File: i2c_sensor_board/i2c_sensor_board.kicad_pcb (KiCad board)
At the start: 2 copper layers, 18 parts, among them J1 Conn_01x03_Pin, J2 Conn_01x04_Pin, J3 Conn_01x04_Pin, SW1 SW_Push, U1 STM32G030K8Tx, U2 BME280, U3 TLV75533PDBV, U4 SN74LV1T34DBV

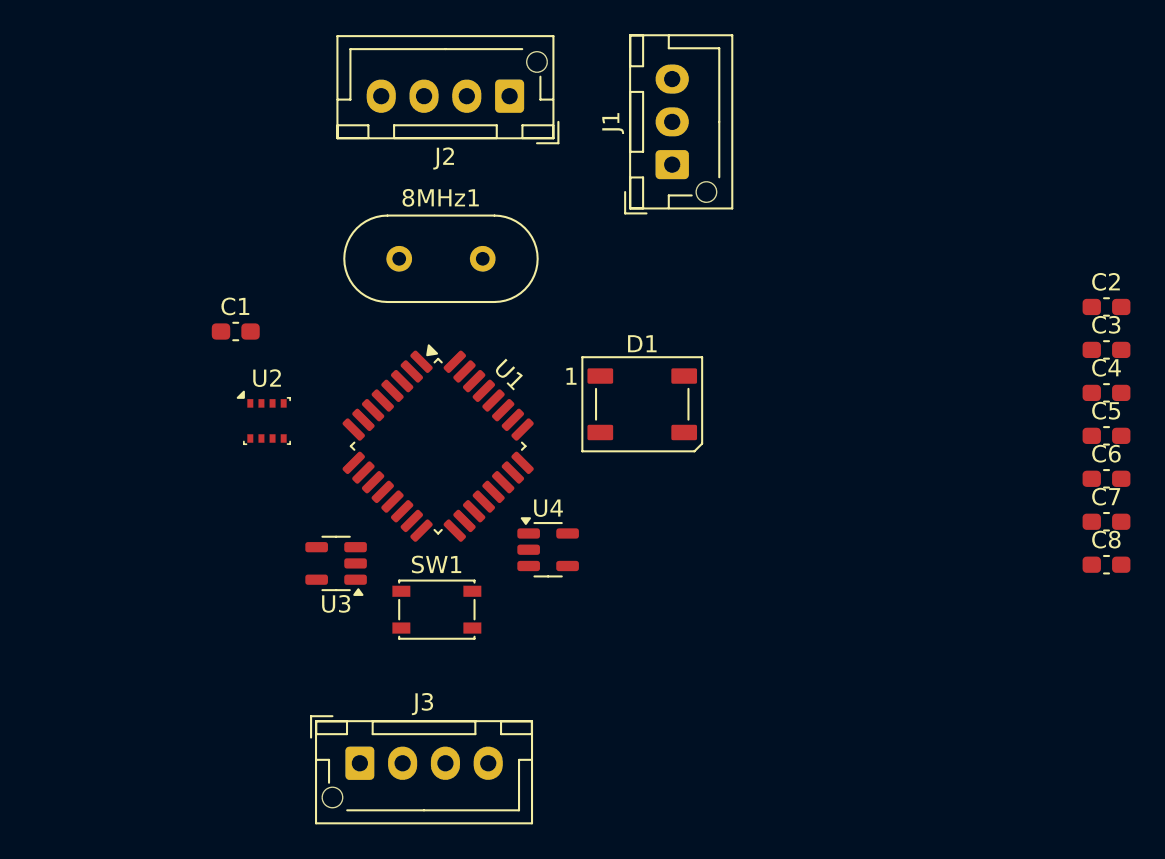
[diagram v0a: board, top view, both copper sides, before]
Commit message: Lots of changes
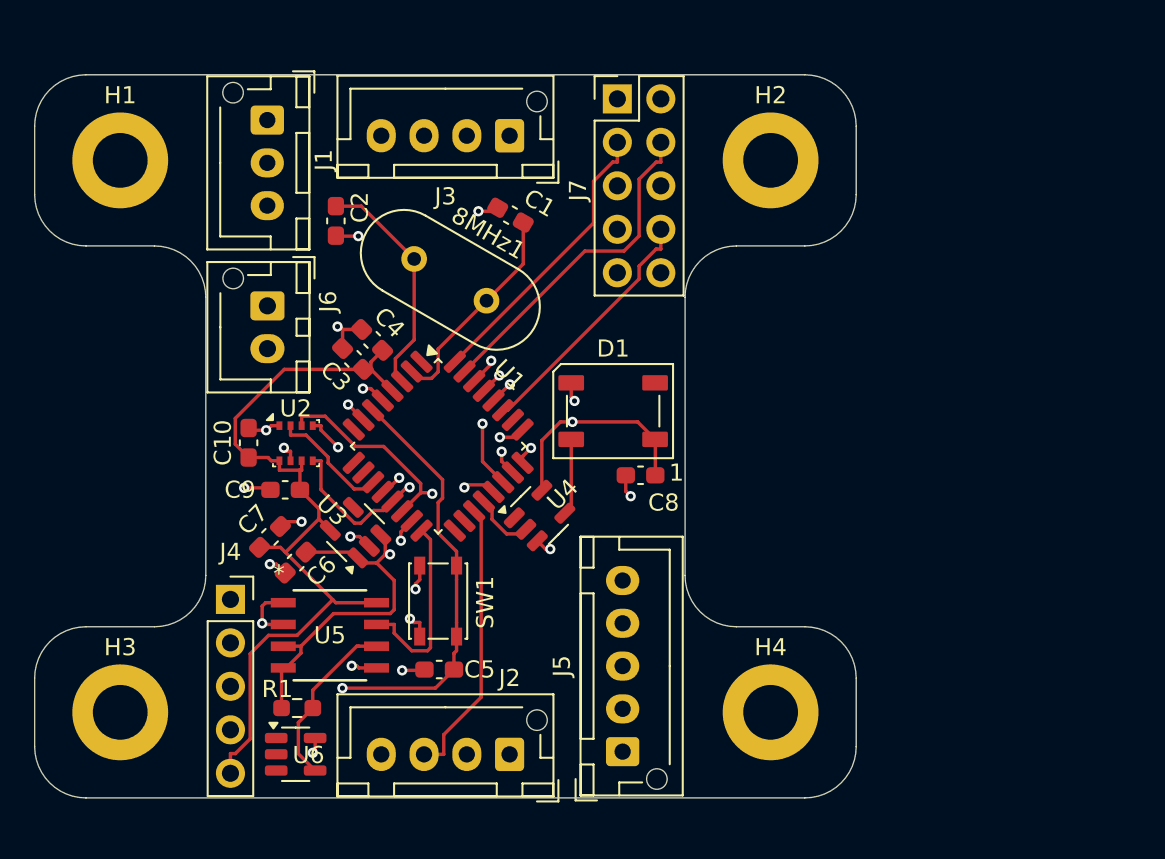
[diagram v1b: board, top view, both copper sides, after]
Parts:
- added C10: 100nF, Capacitor_SMD:C_0603_1608Metric_Pad1.08x0.95mm_HandSolder, F.Cu at (128.5, 79.5)
- added C9: 100nF, Capacitor_SMD:C_0603_1608Metric_Pad1.08x0.95mm_HandSolder, F.Cu at (130.6, 82.2)
- added H1: MountingHole_Pad, MountingHole:MountingHole_3.2mm_M3_DIN965_Pad, F.Cu at (121.0, 63.0)
- added H2: MountingHole_Pad, MountingHole:MountingHole_3.2mm_M3_DIN965_Pad, F.Cu at (159.0, 63.0)
- added H3: MountingHole_Pad, MountingHole:MountingHole_3.2mm_M3_DIN965_Pad, F.Cu at (121.0, 95.2)
- added H4: MountingHole_Pad, MountingHole:MountingHole_3.2mm_M3_DIN965_Pad, F.Cu at (159.0, 95.2)
- added J4: Conn_01x05_Pin, Connector_PinSocket_2.54mm:PinSocket_1x05_P2.54mm_Vertical, F.Cu at (127.4, 88.7)
- added J5: Conn_01x05_Pin, Connector_JST:JST_XH_B5B-XH-AM_1x05_P2.50mm_Vertical, F.Cu at (150.4, 97.5)
- added J6: Conn_01x02_Pin, Connector_JST:JST_XH_B2B-XH-AM_1x02_P2.50mm_Vertical, F.Cu at (129.6, 71.5)
- added J7: Conn_02x05_Counter_Clockwise, Connector_PinHeader_2.54mm:PinHeader_2x05_P2.54mm_Vertical, F.Cu at (150.0, 59.4)
- added R1: 20K, Resistor_SMD:R_0603_1608Metric_Pad0.98x0.95mm_HandSolder, F.Cu at (131.3, 95.0)
- added U5: TMCS1100A2QDR, KiCADv6:SOIC8_D_TEX, F.Cu at (133.2, 90.8)
- added U6: LM4030-2.5, Package_TO_SOT_SMD:SOT-23-5, F.Cu at (131.2, 97.7)
- moved C7 48.9 mm to (129.8, 85.0), turned to 45 degrees
- moved C6 47.6 mm to (131.2, 86.5), turned to -135 degrees
- moved C2 45.3 mm to (133.6, 66.5), turned to 90 degrees
- moved C3 44.0 mm to (134.6, 74.6), turned to 135 degrees
- moved C4 43.0 mm to (135.7, 73.5), turned to -45 degrees
- moved C5 41.3 mm to (139.6, 92.8)
- moved J2 38.5 mm to (143.8, 97.7)
- moved J3 37.7 mm to (143.8, 61.6), turned to 180 degrees
- moved C8 27.7 mm to (151.4, 81.4)
- moved J1 23.8 mm to (129.6, 60.6), turned to -90 degrees
- moved C1 17.4 mm to (143.8, 66.2), turned to -30 degrees
- moved U2 2.14 mm to (131.3, 79.5)
- moved U3 2.13 mm to (134.8, 84.8), turned to 135 degrees
- moved U4 2.06 mm to (145.5, 83.8), turned to 45 degrees
- moved D1 1.75 mm to (149.8, 77.7), turned to 180 degrees
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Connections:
- net Net-(U1-NRST) renamed NRST
- J1 pad 1: unconnected-(J1-Pin_1-Pad1) -> GND
- J1 pad 2: unconnected-(J1-Pin_2-Pad2) -> GPIO_SENS
- J1 pad 3: unconnected-(J1-Pin_3-Pad3) -> +5V
- J2 pad 4: +5V -> Input 5V
- J3 pad 4: +5V -> Input 5V
- U1 pad 11: NSS -> CS1
- U1 pad 15: unconnected-(U1-PB0-Pad15) -> CS2
- U1 pad 16: unconnected-(U1-PB1-Pad16) -> CurrentAnalog
- U1 pad 22: unconnected-(U1-PA11/PA9-Pad22) -> PA11/PA9
- U1 pad 23: unconnected-(U1-PA12/PA10-Pad23) -> PA12/PA10
- U1 pad 24: unconnected-(U1-PA13-Pad24) -> SWDIO
- U1 pad 25: unconnected-(U1-PA14-Pad25) -> SWCLK
- U1 pad 27: unconnected-(U1-PB3-Pad27) -> PB3
- U1 pad 28: unconnected-(U1-PB4-Pad28) -> PB4
- U1 pad 29: unconnected-(U1-PB5-Pad29) -> PB5
- U1 pad 30: unconnected-(U1-PB6-Pad30) -> PB6
- U1 pad 31: unconnected-(U1-PB7-Pad31) -> PB7
- U1 pad 32: unconnected-(U1-PB8-Pad32) -> PB8
- U1 pad 7: unconnected-(U1-PA0-Pad7) -> GPIO_SENS
- U2 pad 1: unconnected-(U2-GND-Pad1) -> GND
- U2 pad 2: unconnected-(U2-CSB-Pad2) -> CS1
- U2 pad 3: unconnected-(U2-SDI-Pad3) -> MOSI
- U2 pad 4: unconnected-(U2-SCK-Pad4) -> SCK
- U2 pad 5: unconnected-(U2-SDO-Pad5) -> MISO
- U2 pad 6: unconnected-(U2-VDDIO-Pad6) -> +3.3V
- U2 pad 7: unconnected-(U2-GND-Pad7) -> GND
- U2 pad 8: unconnected-(U2-VDD-Pad8) -> +3.3V
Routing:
- net +5V: track 0.00 -> 92.7 mm, vias 0 -> 2
- net SCL: track 0.00 -> 54.9 mm
- net +3.3V: track 0.00 -> 48.1 mm
- net SDA: track 0.00 -> 38.2 mm, vias 0 -> 1
- net NRST: track 0.00 -> 31.0 mm, vias 0 -> 1
- net MOSI: track 0.00 -> 26.2 mm, vias 0 -> 1
- net SCK: track 0.00 -> 25.9 mm, vias 0 -> 2
- net GND: track 0.00 -> 25.1 mm, vias 0 -> 18
- net MISO: track 0.00 -> 23.7 mm, vias 0 -> 1
- net SWDIO: track 0.00 -> 23.0 mm, vias 0 -> 1
- net SWCLK: track 0.00 -> 22.2 mm, vias 0 -> 1
- net PB7: track 0.00 -> 19.6 mm
- net CS2: track 0.00 -> 18.4 mm, vias 0 -> 1
- net GPIO_SENS: track 0.00 -> 17.6 mm, vias 0 -> 1
- net PB8: track 0.00 -> 16.9 mm
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- added copper zone on In1.Cu, net GND
- added copper zone on In4.Cu, net GND
- added copper zone on In3.Cu, net Input 5V
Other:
- board outline added: 48 x 42.2 mm
- copper layers 2 -> 6

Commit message: Groovy stuff soon to be replaced by Yattin
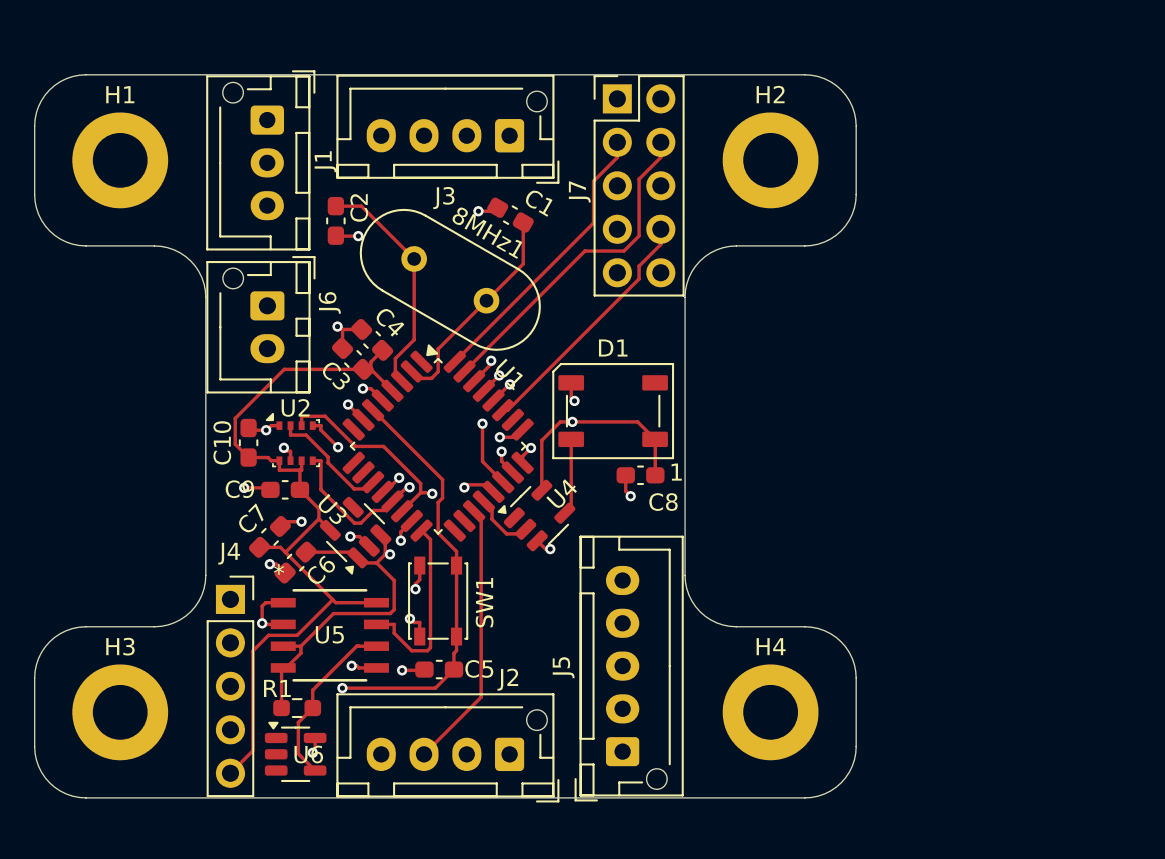
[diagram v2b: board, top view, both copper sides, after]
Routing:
- net SCL: track 54.9 -> 52.8 mm
- net +5V: track 92.7 -> 91.4 mm
